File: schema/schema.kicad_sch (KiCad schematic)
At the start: 12 parts, among them J1 MCU_ATmega328P_Module, J2 MCU_ATmega328P_Module, J3 LCD_1602_I2C, J5 RF_433MHz_TX, SW1 BTN_MORSE, SW2 BTN_SPEED_UP, SW3 BTN_SPEED_DOWN

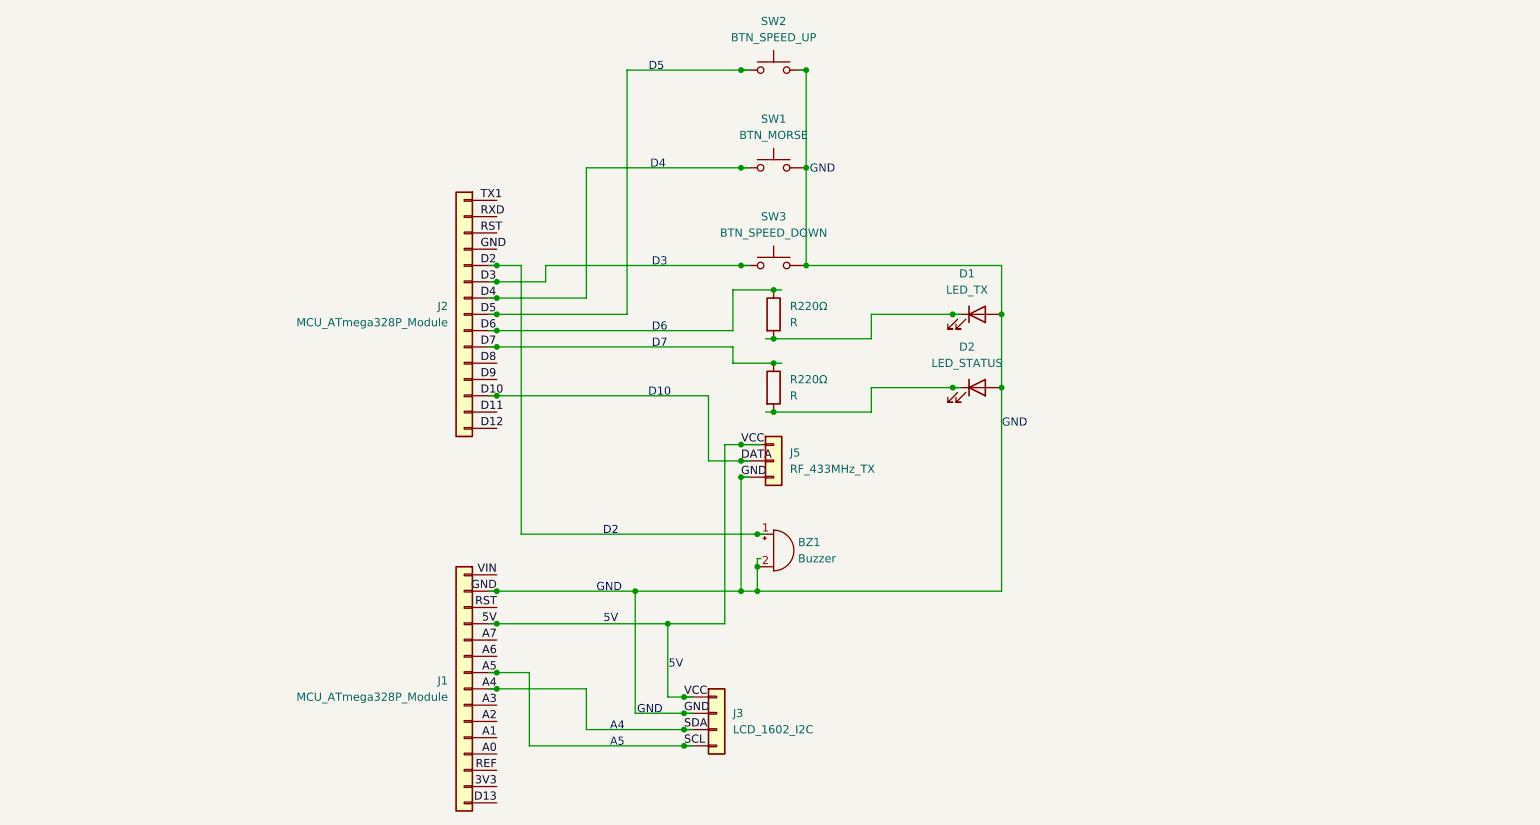
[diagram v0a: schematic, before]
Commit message: Prepare schema for final project
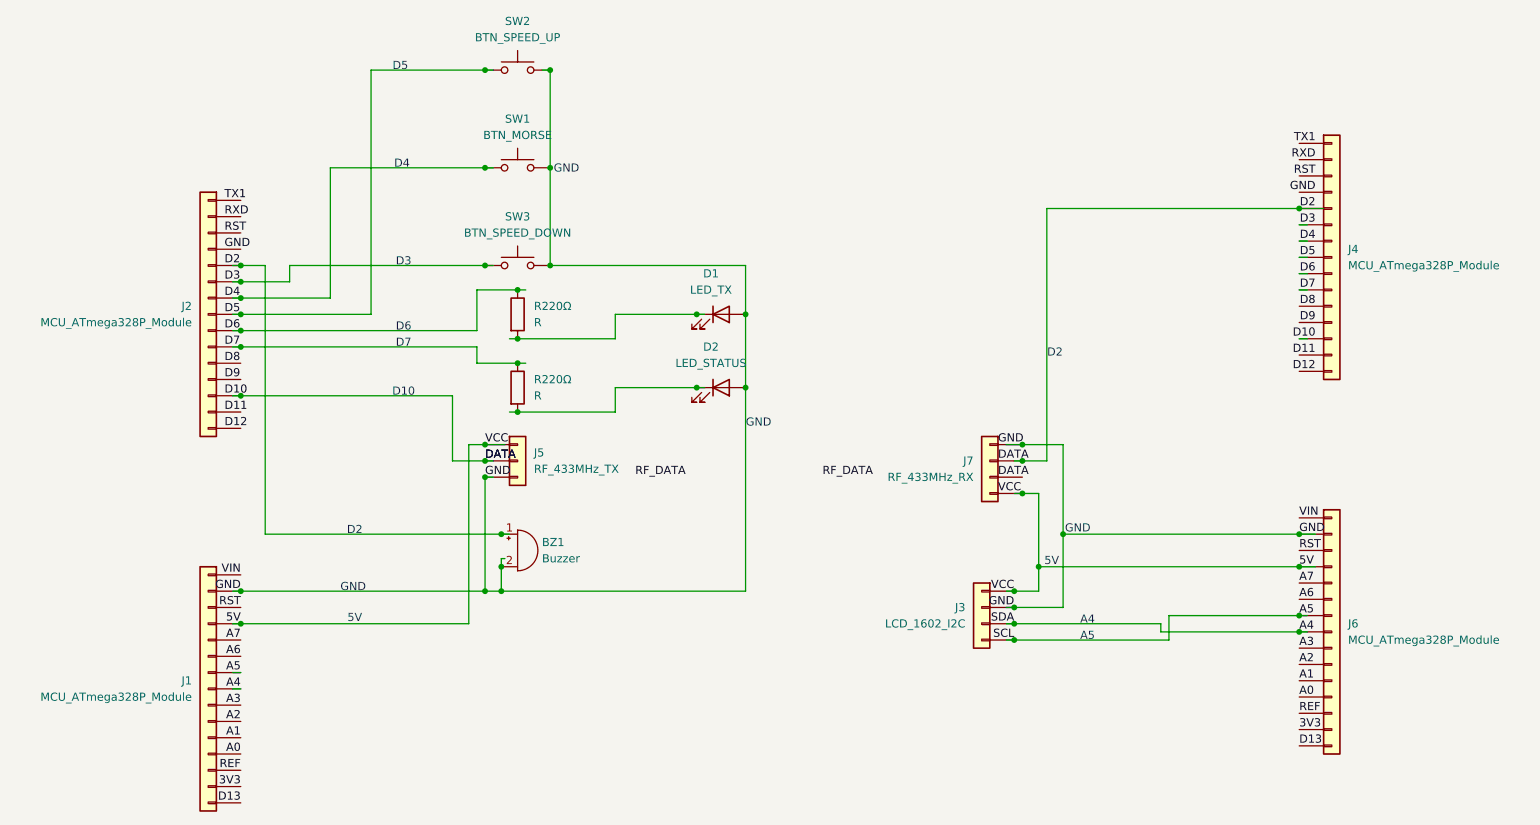
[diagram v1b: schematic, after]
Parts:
- added J4, J6: MCU_ATmega328P_Module, symbol Connector_Generic:Conn_01x15
- added J7: RF_433MHz_RX, symbol Connector_Generic:Conn_01x04
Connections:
- net 3V3: now also J6.14 (Pin_14)
- net 5V: now also J6.4 (Pin_4), J7.4 (Pin_4)
- net A0: now also J6.12 (Pin_12)
- net A1: now also J6.11 (Pin_11)
- net A2: now also J6.10 (Pin_10)
- net A3: now also J6.9 (Pin_9)
- net A4: now also J6.8 (Pin_8)
- net A5: now also J6.7 (Pin_7)
- net A6: now also J6.6 (Pin_6)
- net A7: now also J6.5 (Pin_5)
- net D13: now also J6.15 (Pin_15)
- net D2: now also J4.5 (Pin_5), J7.2 (Pin_2)
- net GND: now also J6.2 (Pin_2), J7.1 (Pin_1)
- net REF: now also J6.13 (Pin_13)
- net RST: now also J6.3 (Pin_3)
- net VIN: now also J6.1 (Pin_1)
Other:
- moved on the sheet: BZ1, D1, D2, J1, J2, J3, J5, R220Ω, SW1, SW2, SW3
